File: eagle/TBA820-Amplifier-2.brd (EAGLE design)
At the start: 30.5 x 25.4 mm, 18 parts, among them IC1 TBA820

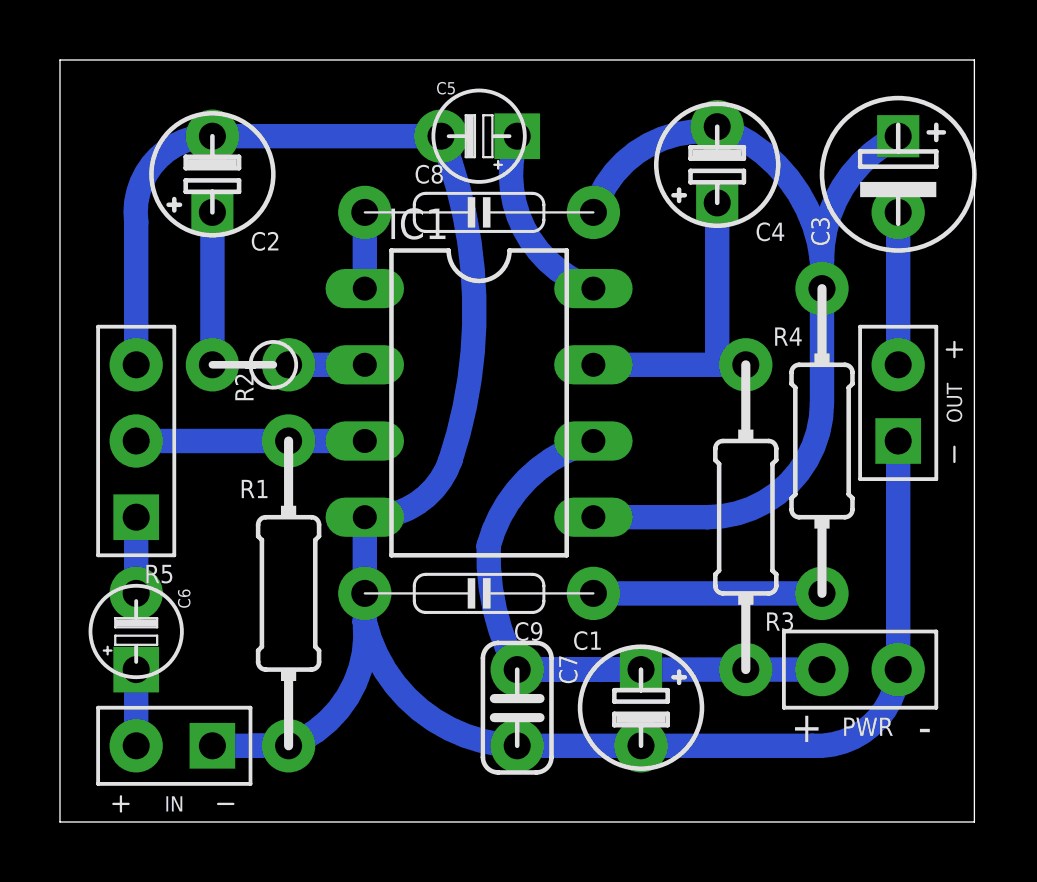
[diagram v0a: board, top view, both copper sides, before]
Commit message: ...
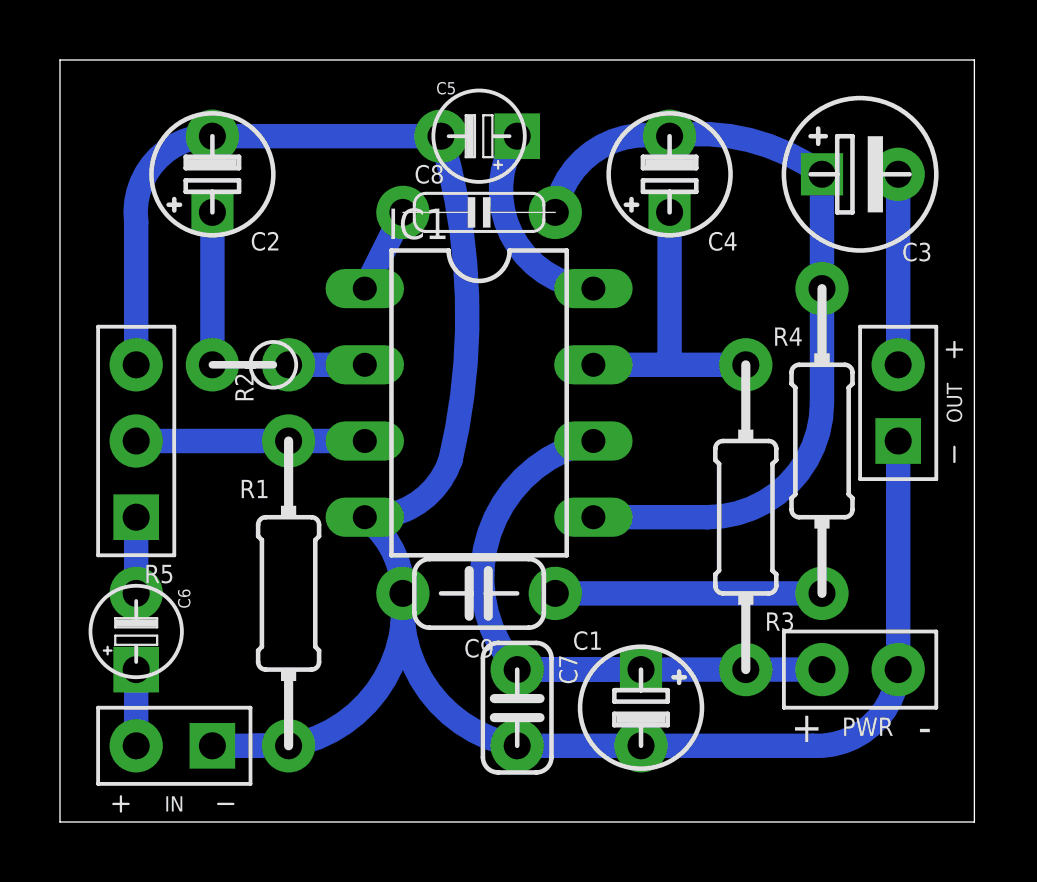
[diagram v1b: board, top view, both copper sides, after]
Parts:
- C8: device c:C075-020X044 -> c:C050-020X044
- C9: device c:C075-020X044 -> c:C050-024X044
- moved C4 1.62 mm to (20.3, 21.6)
- moved C8 1.27 mm to (14.0, 20.3)
- moved C3 1.27 mm to (26.7, 21.6), turned to 180 degrees
- moved C9 1.27 mm to (14.0, 7.62)
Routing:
- net OUT: track 30.6 -> 26.7 mm
- net N$4: track 7.62 -> 8.89 mm
- net N$10: track 5.08 -> 6.35 mm
- net BOOT: track 11.4 -> 10.2 mm
- net VCC: track 23.5 -> 22.3 mm
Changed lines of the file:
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@@
 <setting verticaltext="up"/>
 </settings>
-<grid distance="0.0125" unitdist="inch" unit="inch" style="lines" multiple="8" display="yes" altdistance="0.005" altunitdist="inch" altunit="inch"/>
+<grid distance="0.05" unitdist="inch" unit="inch" style="lines" multiple="2" display="yes" altdistance="0.005" altunitdist="inch" altunit="inch"/>
 <layers>
 <layer number="1" name="Top" color="4" fill="1" visible="no" active="yes"/>
@@
 <layer number="19" name="Unrouted" color="6" fill="1" visible="no" active="yes"/>
 <layer number="20" name="Dimension" color="24" fill="1" visible="yes" active="yes"/>
-<layer number="21" name="tPlace" color="16" fill="1" visible="no" active="yes"/>
+<layer number="21" name="tPlace" color="16" fill="1" visible="yes" active="yes"/>
 <layer number="22" name="bPlace" color="14" fill="1" visible="no" active="yes"/>
-<layer number="23" name="tOrigins" color="15" fill="1" visible="no" active="yes"/>
+<layer number="23" name="tOrigins" color="15" fill="1" visible="yes" active="yes"/>
 <layer number="24" name="bOrigins" color="15" fill="1" visible="no" active="yes"/>
-<layer number="25" name="tNames" color="7" fill="1" visible="no" active="yes"/>
+<layer number="25" name="tNames" color="7" fill="1" visible="yes" active="yes"/>
 <layer number="26" name="bNames" color="7" fill="1" visible="no" active="yes"/>
-<layer number="27" name="tValues" color="7" fill="1" visible="no" active="yes"/>
+<layer number="27" name="tValues" color="7" fill="1" visible="yes" active="yes"/>
 <layer number="28" name="bValues" color="7" fill="1" visible="no" active="yes"/>
 <layer number="29" name="tStop" color="7" fill="3" visible="no" active="yes"/>
@@
 <element name="C1" library="c" package="E2.5-4/V" value="100μF" x="19.3675" y="3.81"/>
 <element name="C2" library="c" package="E2.5-4/V" value="100μF" x="5.08" y="21.59" rot="R180"/>
-<element name="C3" library="c" package="E2,5-5" value="220μF" x="27.94" y="21.59" rot="R90"/>
-<element name="C4" library="c" package="E2.5-4/V" value="100μF" x="21.9075" y="21.9075" rot="R180"/>
+<element name="C3" library="c" package="E2,5-5" value="220μF" x="26.67" y="21.59" rot="R180"/>
+<element name="C4" library="c" package="E2.5-4/V" value="100μF" x="20.32" y="21.59" rot="R180"/>
 <element name="C5" library="c" package="E2,5-3" value="47μF" x="13.97" y="22.86" rot="R180"/>
 <element name="C6" library="c" package="E2,5-3" value="10μF" x="2.54" y="6.35" rot="R90"/>
 <element name="C7" library="c" package="C025-024X044" value="100nF" x="15.24" y="3.81" rot="R270"/>
-<element name="C8" library="c" package="C075-020X044" value="220pF" x="12.7" y="20.32"/>
-<element name="C9" library="c" package="C075-020X044" value="220nF" x="15.24" y="7.62" rot="R180"/>
+<element name="C8" library="c" package="C050-020X044" value="220pF" x="13.97" y="20.32"/>
+<element name="C9" library="c" package="C050-024X044" value="220nF" x="13.97" y="7.62" rot="R180"/>
 <element name="IC1" library="ic" package="DIL08" value="TBA820" x="13.97" y="13.97"/>
 <element name="IN" library="pad" package="SPAD-+" value="SPAD+--+" x="3.81" y="2.54" rot="R90"/>
@@
 <contactref element="C9" pad="1"/>
 <contactref element="R4" pad="2"/>
-<wire x1="25.4" y1="7.62" x2="17.78" y2="7.62" width="0.8128" layer="16"/>
+<wire x1="25.4" y1="7.62" x2="16.51" y2="7.62" width="0.8128" layer="16"/>
 </signal>
 <signal name="N$5">
@@
 <via x="19.3675" y="2.54" extent="1-16" drill="0.381"/>
 <wire x1="10.16" y1="10.16" x2="13.0175" y2="12.065" width="0.8128" layer="16" curve="75"/>
-<wire x1="13.0175" y1="12.065" x2="12.7" y2="22.86" width="0.8128" layer="16" curve="39.921239"/>
+<wire x1="13.0175" y1="12.065" x2="12.7" y2="22.86" width="0.8128" layer="16" curve="30"/>
 <wire x1="12.7" y1="22.86" x2="5.08" y2="22.86" width="0.8128" layer="16"/>
 <contactref element="IC1" pad="4"/>
@@
 <contactref element="IN" pad="1"/>
 <contactref element="C9" pad="2"/>
-<wire x1="10.16" y1="7.62" x2="10.16" y2="10.16" width="0.8128" layer="16"/>
+<wire x1="11.43" y1="7.62" x2="10.16" y2="10.16" width="0.8128" layer="16" curve="53.130102"/>
 <wire x1="7.62" y1="2.54" x2="6.35" y2="2.54" width="0.8128" layer="16"/>
 <wire x1="7.62" y1="2.54" x2="5.08" y2="2.54" width="0.8128" layer="16"/>
@@
 <wire x1="25.0825" y1="2.54" x2="27.94" y2="5.08" width="0.8128" layer="16" curve="90"/>
 <wire x1="27.94" y1="5.08" x2="27.94" y2="12.7" width="0.8128" layer="16"/>
-<wire x1="7.62" y1="2.54" x2="10.16" y2="6.6675" width="0.8128" layer="16" curve="75"/>
-<wire x1="10.16" y1="6.6675" x2="10.16" y2="7.62" width="0.8128" layer="16"/>
-<wire x1="10.16" y1="6.6675" x2="15.24" y2="2.54" width="0.8128" layer="16" curve="75"/>
+<wire x1="7.62" y1="2.54" x2="11.43" y2="6.6675" width="0.8128" layer="16" curve="75"/>
+<wire x1="11.43" y1="6.6675" x2="11.43" y2="7.62" width="0.8128" layer="16"/>
+<wire x1="11.43" y1="6.6675" x2="15.24" y2="2.54" width="0.8128" layer="16" curve="75"/>
 <wire x1="19.3675" y1="2.54" x2="25.0825" y2="2.54" width="0.8128" layer="16"/>
 </signal>
@@
 <contactref element="IC1" pad="8"/>
 <contactref element="C5" pad="+"/>
-<wire x1="15.24" y1="22.86" x2="17.78" y2="17.78" width="0.8128" layer="16" curve="90"/>
+<wire x1="15.24" y1="22.86" x2="17.78" y2="17.78" width="0.8128" layer="16" curve="120"/>
 </signal>
 <signal name="FREQ">
 <contactref element="C8" pad="1"/>
 <contactref element="IC1" pad="1"/>
-<wire x1="10.16" y1="20.32" x2="10.16" y2="17.78" width="0.8128" layer="16"/>
+<wire x1="11.43" y1="20.32" x2="10.16" y2="17.78" width="0.8128" layer="16"/>
 </signal>
 <signal name="OUT">
@@
 <wire x1="21.59" y1="10.16" x2="25.4" y2="13.97" width="0.8128" layer="16" curve="90"/>
 <wire x1="25.4" y1="13.97" x2="25.4" y2="17.78" width="0.8128" layer="16"/>
-<wire x1="21.9075" y1="23.1775" x2="22.5425" y2="22.86" width="0.8128" layer="16"/>
-<wire x1="22.5425" y1="22.86" x2="17.78" y2="20.32" width="0.8128" layer="16" curve="90"/>
-<wire x1="21.9075" y1="23.1775" x2="25.4" y2="18.7325" width="0.8128" layer="16" curve="-63.215004"/>
-<wire x1="27.94" y1="22.86" x2="25.4" y2="18.7325" width="0.8128" layer="16" curve="63.215004"/>
-<wire x1="25.4" y1="18.7325" x2="25.4" y2="17.78" width="0.8128" layer="16"/>
+<wire x1="20.32" y1="22.86" x2="20.0025" y2="22.86" width="0.8128" layer="16"/>
+<wire x1="20.0025" y1="22.86" x2="16.51" y2="20.32" width="0.8128" layer="16" curve="90"/>
+<wire x1="20.32" y1="22.86" x2="25.4" y2="21.59" width="0.8128" layer="16" curve="-45"/>
+<wire x1="25.4" y1="21.59" x2="25.4" y2="17.78" width="0.8128" layer="16"/>
 </signal>
 <signal name="N$10">
 <contactref element="C3" pad="-"/>
 <contactref element="OUT" pad="2"/>
-<wire x1="27.94" y1="15.24" x2="27.94" y2="20.32" width="0.8128" layer="16"/>
+<wire x1="27.94" y1="15.24" x2="27.94" y2="21.59" width="0.8128" layer="16"/>
 </signal>
 <signal name="N$11">
@@
 <contactref element="IC1" pad="7"/>
 <contactref element="C4" pad="+"/>
-<wire x1="22.86" y1="15.24" x2="17.78" y2="15.24" width="0.8128" layer="16"/>
-<wire x1="21.9075" y1="20.6375" x2="21.9075" y2="15.24" width="0.8128" layer="16"/>
-<wire x1="21.9075" y1="15.24" x2="22.86" y2="15.24" width="0.8128" layer="16"/>
+<wire x1="20.32" y1="15.24" x2="17.78" y2="15.24" width="0.8128" layer="16"/>
+<wire x1="20.32" y1="20.32" x2="20.32" y2="15.24" width="0.8128" layer="16"/>
+<wire x1="20.32" y1="15.24" x2="22.86" y2="15.24" width="0.8128" layer="16"/>
 </signal>
 <signal name="VCC">
@@
 <contactref element="R3" pad="1"/>
 <contactref element="C1" pad="+"/>
-<wire x1="17.78" y1="12.7" x2="14.2875" y2="9.2075" width="0.8128" layer="16" curve="60"/>
+<wire x1="17.78" y1="12.7" x2="15.24" y2="5.08" width="0.8128" layer="16" curve="120"/>
 <via x="19.3675" y="5.08" extent="1-16" drill="0.381"/>
 <wire x1="19.3675" y1="5.08" x2="15.24" y2="5.08" width="0.8128" layer="16"/>
 <wire x1="15.24" y1="5.08" x2="22.86" y2="5.08" width="0.8128" layer="16"/>
 <wire x1="22.86" y1="5.08" x2="25.4" y2="5.08" width="0.8128" layer="16"/>
-<wire x1="14.2875" y1="9.2075" x2="15.24" y2="5.08" width="0.8128" layer="16" curve="30"/>
 </signal>
 </signals>

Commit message: ...
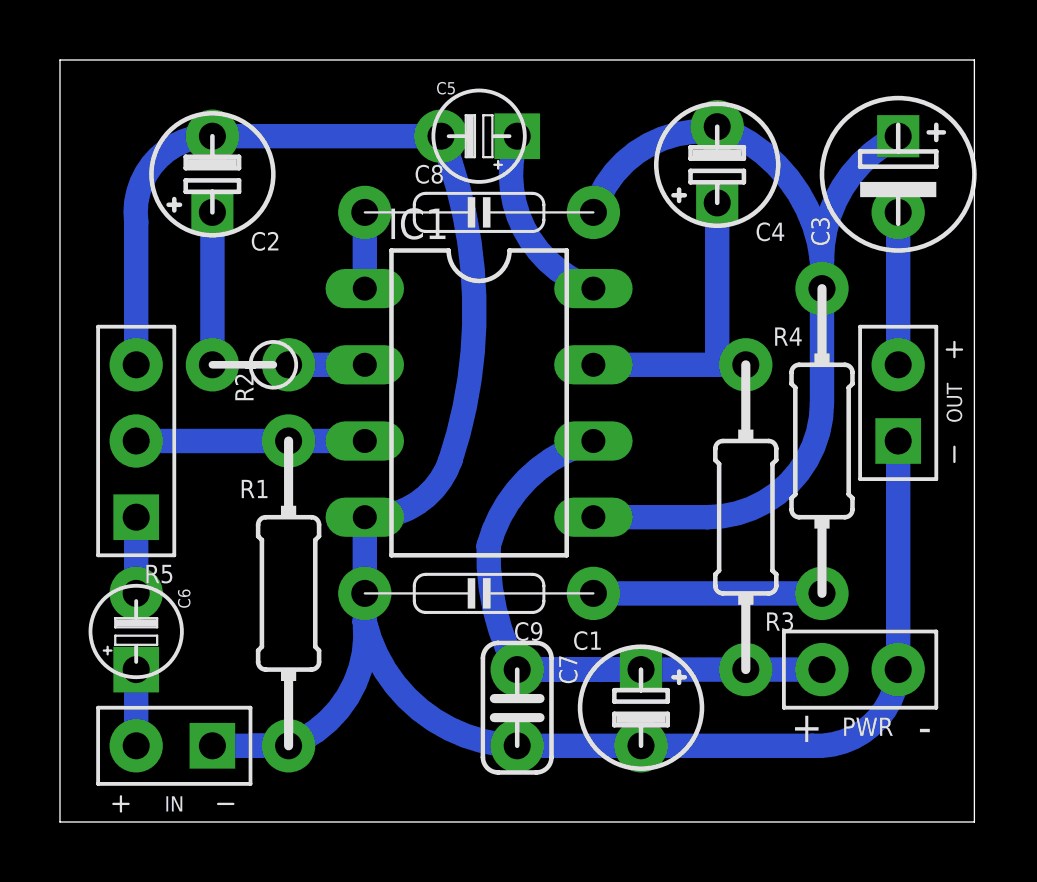
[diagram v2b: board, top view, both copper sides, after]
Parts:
- C8: device c:C050-020X044 -> c:C075-020X044
- C9: device c:C050-024X044 -> c:C075-020X044
- moved C4 1.62 mm to (21.9, 21.9)
- moved C8 1.27 mm to (12.7, 20.3)
- moved C3 1.27 mm to (27.9, 21.6), turned to 90 degrees
- moved C9 1.27 mm to (15.2, 7.62)
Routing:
- net OUT: track 26.7 -> 30.6 mm
- net N$4: track 8.89 -> 7.62 mm
- net N$10: track 6.35 -> 5.08 mm
- net BOOT: track 10.2 -> 11.4 mm
- net VCC: track 22.3 -> 23.5 mm
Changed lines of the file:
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@@
 <setting verticaltext="up"/>
 </settings>
-<grid distance="0.05" unitdist="inch" unit="inch" style="lines" multiple="2" display="yes" altdistance="0.005" altunitdist="inch" altunit="inch"/>
+<grid distance="0.0125" unitdist="inch" unit="inch" style="lines" multiple="8" display="yes" altdistance="0.005" altunitdist="inch" altunit="inch"/>
 <layers>
 <layer number="1" name="Top" color="4" fill="1" visible="no" active="yes"/>
@@
 <layer number="19" name="Unrouted" color="6" fill="1" visible="no" active="yes"/>
 <layer number="20" name="Dimension" color="24" fill="1" visible="yes" active="yes"/>
-<layer number="21" name="tPlace" color="16" fill="1" visible="yes" active="yes"/>
+<layer number="21" name="tPlace" color="16" fill="1" visible="no" active="yes"/>
 <layer number="22" name="bPlace" color="14" fill="1" visible="no" active="yes"/>
-<layer number="23" name="tOrigins" color="15" fill="1" visible="yes" active="yes"/>
+<layer number="23" name="tOrigins" color="15" fill="1" visible="no" active="yes"/>
 <layer number="24" name="bOrigins" color="15" fill="1" visible="no" active="yes"/>
-<layer number="25" name="tNames" color="7" fill="1" visible="yes" active="yes"/>
+<layer number="25" name="tNames" color="7" fill="1" visible="no" active="yes"/>
 <layer number="26" name="bNames" color="7" fill="1" visible="no" active="yes"/>
-<layer number="27" name="tValues" color="7" fill="1" visible="yes" active="yes"/>
+<layer number="27" name="tValues" color="7" fill="1" visible="no" active="yes"/>
 <layer number="28" name="bValues" color="7" fill="1" visible="no" active="yes"/>
 <layer number="29" name="tStop" color="7" fill="3" visible="no" active="yes"/>
@@
 <element name="C1" library="c" package="E2.5-4/V" value="100μF" x="19.3675" y="3.81"/>
 <element name="C2" library="c" package="E2.5-4/V" value="100μF" x="5.08" y="21.59" rot="R180"/>
-<element name="C3" library="c" package="E2,5-5" value="220μF" x="26.67" y="21.59" rot="R180"/>
-<element name="C4" library="c" package="E2.5-4/V" value="100μF" x="20.32" y="21.59" rot="R180"/>
+<element name="C3" library="c" package="E2,5-5" value="220μF" x="27.94" y="21.59" rot="R90"/>
+<element name="C4" library="c" package="E2.5-4/V" value="100μF" x="21.9075" y="21.9075" rot="R180"/>
 <element name="C5" library="c" package="E2,5-3" value="47μF" x="13.97" y="22.86" rot="R180"/>
 <element name="C6" library="c" package="E2,5-3" value="10μF" x="2.54" y="6.35" rot="R90"/>
 <element name="C7" library="c" package="C025-024X044" value="100nF" x="15.24" y="3.81" rot="R270"/>
-<element name="C8" library="c" package="C050-020X044" value="220pF" x="13.97" y="20.32"/>
-<element name="C9" library="c" package="C050-024X044" value="220nF" x="13.97" y="7.62" rot="R180"/>
+<element name="C8" library="c" package="C075-020X044" value="220pF" x="12.7" y="20.32"/>
+<element name="C9" library="c" package="C075-020X044" value="220nF" x="15.24" y="7.62" rot="R180"/>
 <element name="IC1" library="ic" package="DIL08" value="TBA820" x="13.97" y="13.97"/>
 <element name="IN" library="pad" package="SPAD-+" value="SPAD+--+" x="3.81" y="2.54" rot="R90"/>
@@
 <contactref element="C9" pad="1"/>
 <contactref element="R4" pad="2"/>
-<wire x1="25.4" y1="7.62" x2="16.51" y2="7.62" width="0.8128" layer="16"/>
+<wire x1="25.4" y1="7.62" x2="17.78" y2="7.62" width="0.8128" layer="16"/>
 </signal>
 <signal name="N$5">
@@
 <via x="19.3675" y="2.54" extent="1-16" drill="0.381"/>
 <wire x1="10.16" y1="10.16" x2="13.0175" y2="12.065" width="0.8128" layer="16" curve="75"/>
-<wire x1="13.0175" y1="12.065" x2="12.7" y2="22.86" width="0.8128" layer="16" curve="30"/>
+<wire x1="13.0175" y1="12.065" x2="12.7" y2="22.86" width="0.8128" layer="16" curve="39.921239"/>
 <wire x1="12.7" y1="22.86" x2="5.08" y2="22.86" width="0.8128" layer="16"/>
 <contactref element="IC1" pad="4"/>
@@
 <contactref element="IN" pad="1"/>
 <contactref element="C9" pad="2"/>
-<wire x1="11.43" y1="7.62" x2="10.16" y2="10.16" width="0.8128" layer="16" curve="53.130102"/>
+<wire x1="10.16" y1="7.62" x2="10.16" y2="10.16" width="0.8128" layer="16"/>
 <wire x1="7.62" y1="2.54" x2="6.35" y2="2.54" width="0.8128" layer="16"/>
 <wire x1="7.62" y1="2.54" x2="5.08" y2="2.54" width="0.8128" layer="16"/>
@@
 <wire x1="25.0825" y1="2.54" x2="27.94" y2="5.08" width="0.8128" layer="16" curve="90"/>
 <wire x1="27.94" y1="5.08" x2="27.94" y2="12.7" width="0.8128" layer="16"/>
-<wire x1="7.62" y1="2.54" x2="11.43" y2="6.6675" width="0.8128" layer="16" curve="75"/>
-<wire x1="11.43" y1="6.6675" x2="11.43" y2="7.62" width="0.8128" layer="16"/>
-<wire x1="11.43" y1="6.6675" x2="15.24" y2="2.54" width="0.8128" layer="16" curve="75"/>
+<wire x1="7.62" y1="2.54" x2="10.16" y2="6.6675" width="0.8128" layer="16" curve="75"/>
+<wire x1="10.16" y1="6.6675" x2="10.16" y2="7.62" width="0.8128" layer="16"/>
+<wire x1="10.16" y1="6.6675" x2="15.24" y2="2.54" width="0.8128" layer="16" curve="75"/>
 <wire x1="19.3675" y1="2.54" x2="25.0825" y2="2.54" width="0.8128" layer="16"/>
 </signal>
@@
 <contactref element="IC1" pad="8"/>
 <contactref element="C5" pad="+"/>
-<wire x1="15.24" y1="22.86" x2="17.78" y2="17.78" width="0.8128" layer="16" curve="120"/>
+<wire x1="15.24" y1="22.86" x2="17.78" y2="17.78" width="0.8128" layer="16" curve="90"/>
 </signal>
 <signal name="FREQ">
 <contactref element="C8" pad="1"/>
 <contactref element="IC1" pad="1"/>
-<wire x1="11.43" y1="20.32" x2="10.16" y2="17.78" width="0.8128" layer="16"/>
+<wire x1="10.16" y1="20.32" x2="10.16" y2="17.78" width="0.8128" layer="16"/>
 </signal>
 <signal name="OUT">
@@
 <wire x1="21.59" y1="10.16" x2="25.4" y2="13.97" width="0.8128" layer="16" curve="90"/>
 <wire x1="25.4" y1="13.97" x2="25.4" y2="17.78" width="0.8128" layer="16"/>
-<wire x1="20.32" y1="22.86" x2="20.0025" y2="22.86" width="0.8128" layer="16"/>
-<wire x1="20.0025" y1="22.86" x2="16.51" y2="20.32" width="0.8128" layer="16" curve="90"/>
-<wire x1="20.32" y1="22.86" x2="25.4" y2="21.59" width="0.8128" layer="16" curve="-45"/>
-<wire x1="25.4" y1="21.59" x2="25.4" y2="17.78" width="0.8128" layer="16"/>
+<wire x1="21.9075" y1="23.1775" x2="22.5425" y2="22.86" width="0.8128" layer="16"/>
+<wire x1="22.5425" y1="22.86" x2="17.78" y2="20.32" width="0.8128" layer="16" curve="90"/>
+<wire x1="21.9075" y1="23.1775" x2="25.4" y2="18.7325" width="0.8128" layer="16" curve="-63.215004"/>
+<wire x1="27.94" y1="22.86" x2="25.4" y2="18.7325" width="0.8128" layer="16" curve="63.215004"/>
+<wire x1="25.4" y1="18.7325" x2="25.4" y2="17.78" width="0.8128" layer="16"/>
 </signal>
 <signal name="N$10">
 <contactref element="C3" pad="-"/>
 <contactref element="OUT" pad="2"/>
-<wire x1="27.94" y1="15.24" x2="27.94" y2="21.59" width="0.8128" layer="16"/>
+<wire x1="27.94" y1="15.24" x2="27.94" y2="20.32" width="0.8128" layer="16"/>
 </signal>
 <signal name="N$11">
@@
 <contactref element="IC1" pad="7"/>
 <contactref element="C4" pad="+"/>
-<wire x1="20.32" y1="15.24" x2="17.78" y2="15.24" width="0.8128" layer="16"/>
-<wire x1="20.32" y1="20.32" x2="20.32" y2="15.24" width="0.8128" layer="16"/>
-<wire x1="20.32" y1="15.24" x2="22.86" y2="15.24" width="0.8128" layer="16"/>
+<wire x1="22.86" y1="15.24" x2="17.78" y2="15.24" width="0.8128" layer="16"/>
+<wire x1="21.9075" y1="20.6375" x2="21.9075" y2="15.24" width="0.8128" layer="16"/>
+<wire x1="21.9075" y1="15.24" x2="22.86" y2="15.24" width="0.8128" layer="16"/>
 </signal>
 <signal name="VCC">
@@
 <contactref element="R3" pad="1"/>
 <contactref element="C1" pad="+"/>
-<wire x1="17.78" y1="12.7" x2="15.24" y2="5.08" width="0.8128" layer="16" curve="120"/>
+<wire x1="17.78" y1="12.7" x2="14.2875" y2="9.2075" width="0.8128" layer="16" curve="60"/>
 <via x="19.3675" y="5.08" extent="1-16" drill="0.381"/>
 <wire x1="19.3675" y1="5.08" x2="15.24" y2="5.08" width="0.8128" layer="16"/>
 <wire x1="15.24" y1="5.08" x2="22.86" y2="5.08" width="0.8128" layer="16"/>
 <wire x1="22.86" y1="5.08" x2="25.4" y2="5.08" width="0.8128" layer="16"/>
+<wire x1="14.2875" y1="9.2075" x2="15.24" y2="5.08" width="0.8128" layer="16" curve="30"/>
 </signal>
 </signals>
